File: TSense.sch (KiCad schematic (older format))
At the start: 52 parts, among them U10 LM393M, U11 LM393M, U2 LM393M, U3 LM393M, U4 LM393M, U5 LM393M, U6 LM393M, U7 LM393M, U8 LM393M, U9 LM393M

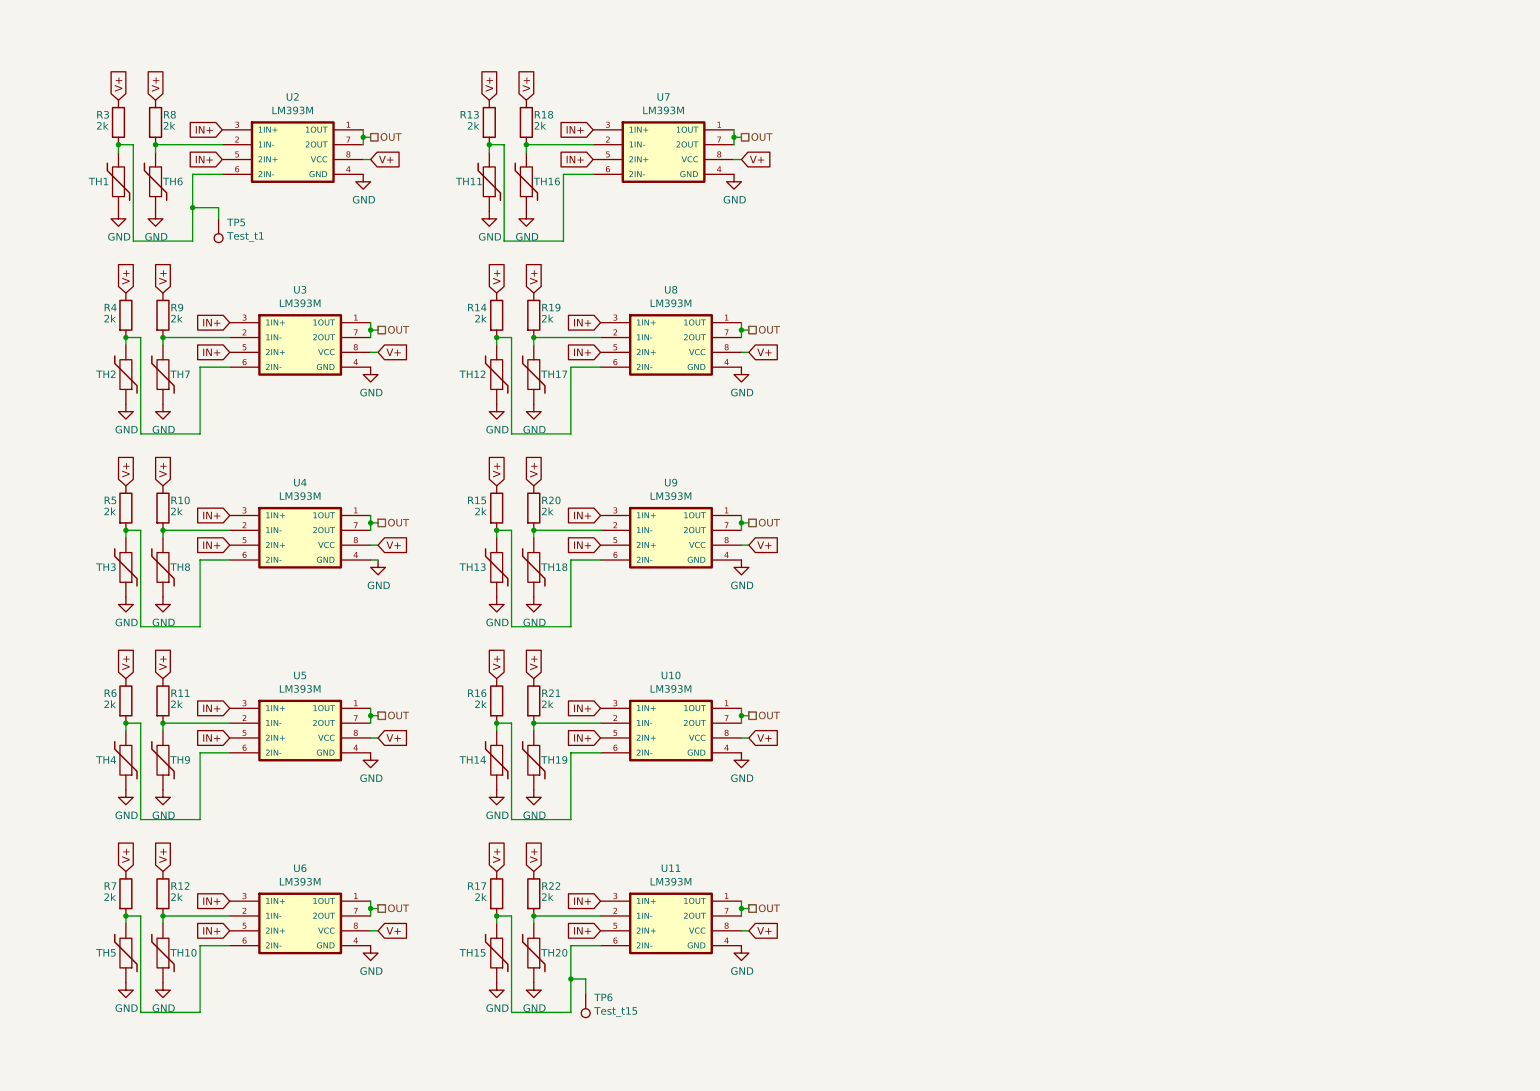
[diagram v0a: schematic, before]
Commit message: new
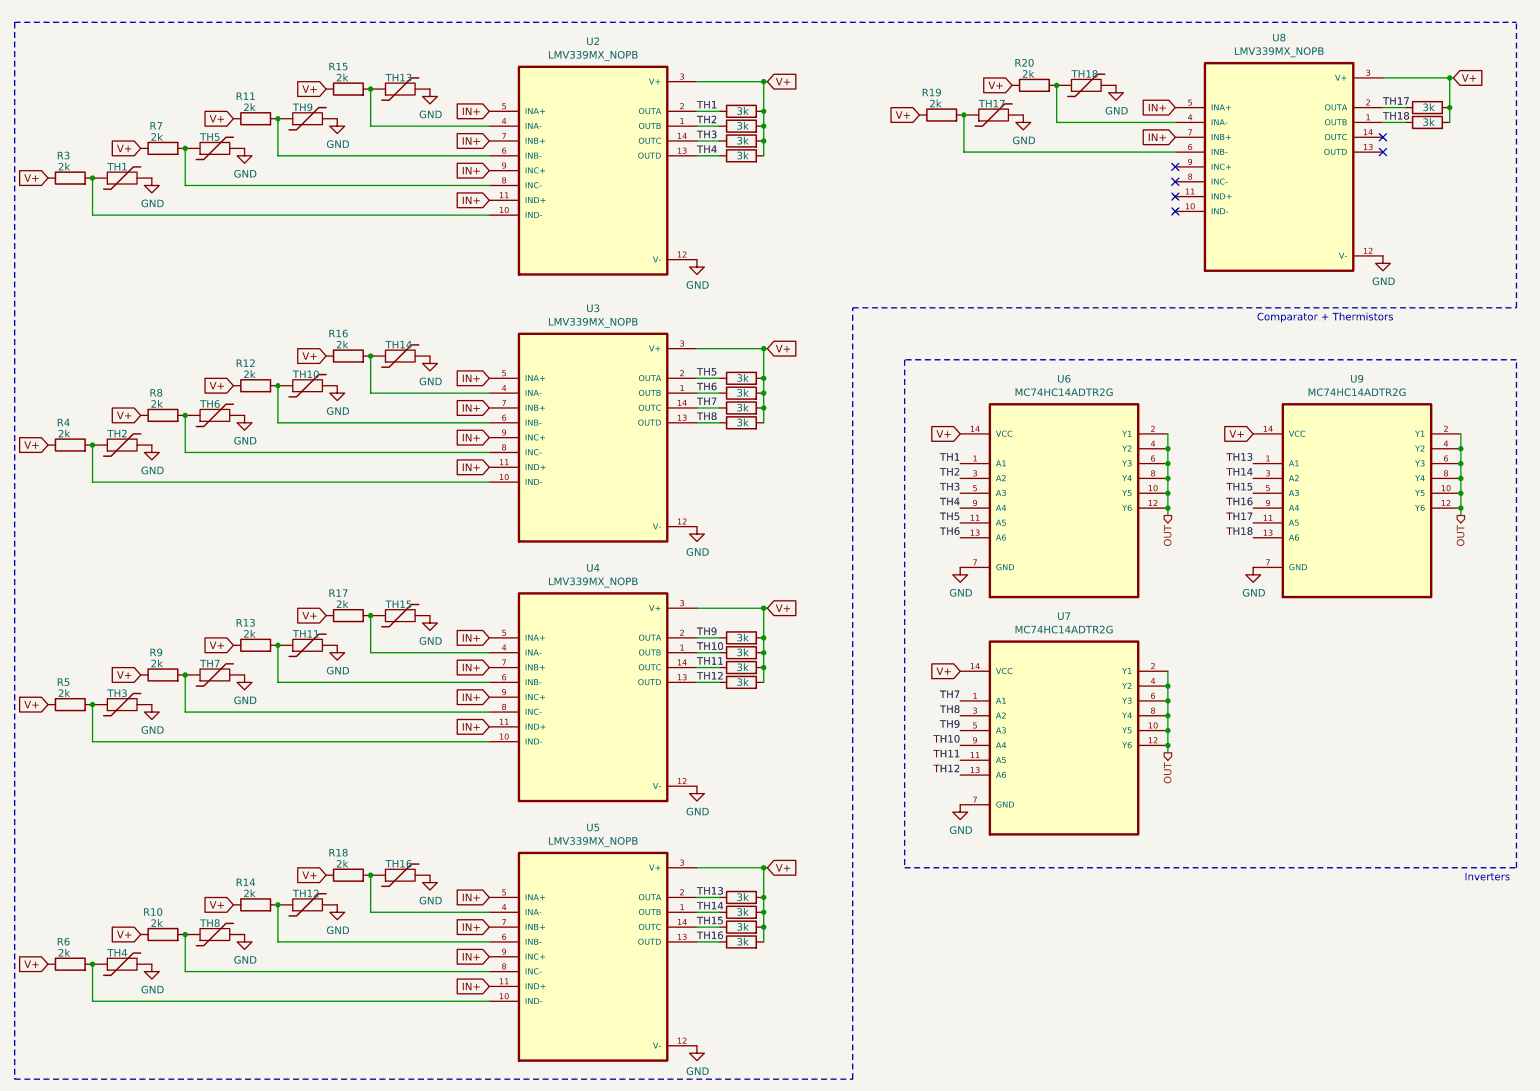
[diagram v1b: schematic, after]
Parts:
- removed R21, R22: 2k, Resistor_SMD:R_0805_2012Metric_Pad1.20x1.40mm_HandSolder, symbol Device:R
- removed TH19, TH20: 1k, Resistor_SMD:R_0603_1608Metric_Pad0.98x0.95mm_HandSolder, symbol Device:Thermistor
- removed TP5: Test_t1, LHRE Footprint Library:Test_Point_Tiny, symbol Connector:TestPoint
- removed TP6: Test_t15, LHRE Footprint Library:Test_Point_Tiny, symbol Connector:TestPoint
- removed U10, U11, U2, U3, U4, U5, U6, U7, U8, U9: LM393M, LHRE Footprint Library:SOIC127P599X175-8N, symbol Comparator:LM393DR
- added R? (x18): 3k, Resistor_SMD:R_0603_1608Metric_Pad0.98x0.95mm_HandSolder, symbol Device:R
- added U2, U3, U4, U5, U8: LMV339MX_NOPB, SOIC127P600X175-14N, symbol Comparator:LMV339MX_NOPB
- added U6, U7, U9: MC74HC14ADTR2G, LHRE Footprint Library:MC74HC14ADTR2G, symbol MC74HCT14ADG:MC74HC14ADTR2G
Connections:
- net GND: now also TH1.2, TH10.2, TH11.2, TH12.2, TH13.2, TH14.2, TH15.2, TH16.2, TH17.2, TH18.2, TH2.2, TH3.2, TH4.2, TH5.2, TH6.2, TH7.2, TH8.2, TH9.2, U2.12 (V-), U3.12 (V-), U4.12 (V-), U5.12 (V-), U6.7 (GND), U7.7 (GND), U8.12 (V-), U9.7 (GND); no longer TH1.1, TH10.1, TH11.1, TH12.1, TH13.1, TH14.1, TH15.1, TH16.1, TH17.1, TH18.1, TH2.1, TH3.1, TH4.1, TH5.1, TH6.1, TH7.1, TH8.1, TH9.1
- net IN+: now also U2.11 (IND+), U2.5 (INA+), U2.7 (INB+), U2.9 (INC+), U3.11 (IND+), U3.5 (INA+), U3.7 (INB+), U3.9 (INC+), U4.11 (IND+), U4.5 (INA+), U4.7 (INB+), U4.9 (INC+), U5.11 (IND+), U5.5 (INA+), U5.7 (INB+), U5.9 (INC+), U8.5 (INA+), U8.7 (INB+)
- net OUT: now also U6.10 (Y5), U6.12 (Y6), U6.2 (Y1), U6.4 (Y2), U6.6 (Y3), U6.8 (Y4), U7.10 (Y5), U7.12 (Y6), U7.2 (Y1), U7.4 (Y2), U7.6 (Y3), U7.8 (Y4), U9.10 (Y5), U9.12 (Y6), U9.2 (Y1), U9.4 (Y2), U9.6 (Y3), U9.8 (Y4)
- net V+: now also R?.2, R?.2, R?.2, R?.2, R?.2, R?.2, R?.2, R?.2, R?.2, R?.2, R?.2, R?.2, R?.2, R?.2, R?.2, R?.2, R?.2, R?.2, U2.3 (V+), U3.3 (V+), U4.3 (V+), U5.3 (V+), U6.14 (VCC), U7.14 (VCC), U8.3 (V+), U9.14 (VCC)
- net at R8.2: now also TH6.1, U3.8 (INC-); no longer TH6.2
- net at R3.2: now also TH1.1, U2.10 (IND-); no longer TH1.2
- net at R4.2: now also TH2.1, U3.10 (IND-); no longer TH2.2
- net at R9.2: now also TH7.1, U4.8 (INC-); no longer TH7.2
- net at R10.2: now also TH8.1, U5.8 (INC-); no longer TH8.2
- net at R5.2: now also TH3.1, U4.10 (IND-); no longer TH3.2
- net at R11.2: now also TH9.1, U2.6 (INB-); no longer TH9.2
- net at R6.2: now also TH4.1, U5.10 (IND-); no longer TH4.2
- net at R12.2: now also TH10.1, U3.6 (INB-); no longer TH10.2
- net at R7.2: now also TH5.1, U2.8 (INC-); no longer TH5.2
- net at R18.2: now also TH16.1, U5.4 (INA-); no longer TH16.2
- net at R13.2: now also TH11.1, U4.6 (INB-); no longer TH11.2
- net at R19.2: now also TH17.1, U8.6 (INB-); no longer TH17.2
- net at R14.2: now also TH12.1, U5.6 (INB-); no longer TH12.2
- net at R20.2: now also TH18.1, U8.4 (INA-); no longer TH18.2
- net at R15.2: now also TH13.1, U2.4 (INA-); no longer TH13.2
- net at R16.2: now also TH14.1, U3.4 (INA-); no longer TH14.2
- net at R17.2: now also TH15.1, U4.4 (INA-); no longer TH15.2
- new net TH1: R?.1, U2.2 (OUTA), U6.1 (A1)
- new net TH10: R?.1, U4.1 (OUTB), U7.9 (A4)
- new net TH11: R?.1, U4.14 (OUTC), U7.11 (A5)
- new net TH12: R?.1, U4.13 (OUTD), U7.13 (A6)
- new net TH13: R?.1, U5.2 (OUTA), U9.1 (A1)
- new net TH14: R?.1, U5.1 (OUTB), U9.3 (A2)
- new net TH15: R?.1, U5.14 (OUTC), U9.5 (A3)
- new net TH16: R?.1, U5.13 (OUTD), U9.9 (A4)
- new net TH17: R?.1, U8.2 (OUTA), U9.11 (A5)
- new net TH18: R?.1, U8.1 (OUTB), U9.13 (A6)
- new net TH2: R?.1, U2.1 (OUTB), U6.3 (A2)
- new net TH3: R?.1, U2.14 (OUTC), U6.5 (A3)
- new net TH4: R?.1, U2.13 (OUTD), U6.9 (A4)
- new net TH5: R?.1, U3.2 (OUTA), U6.11 (A5)
- new net TH6: R?.1, U3.1 (OUTB), U6.13 (A6)
- new net TH7: R?.1, U3.14 (OUTC), U7.1 (A1)
- new net TH8: R?.1, U3.13 (OUTD), U7.3 (A2)
- new net TH9: R?.1, U4.2 (OUTA), U7.5 (A3)
- no-connect marks 0 -> 6
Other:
- note added: "Comparator + Thermistors\n"
- note added: "Inverters\n"

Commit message: Add files via upload
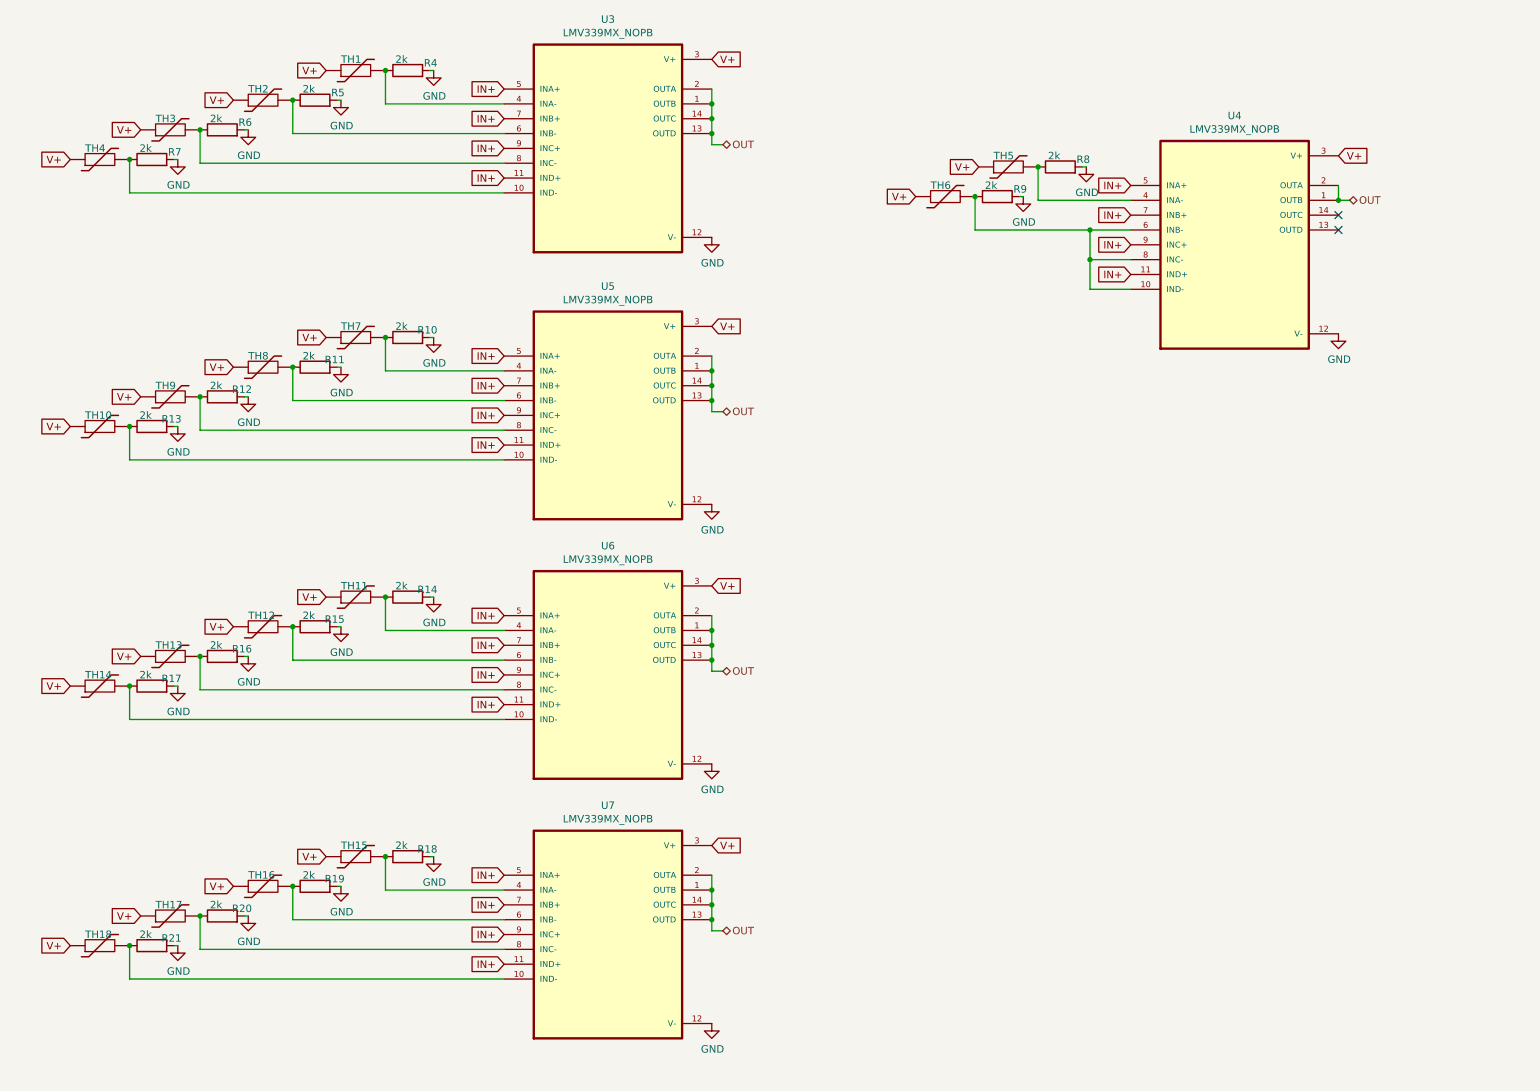
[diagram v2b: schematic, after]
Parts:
- removed R7: 2k, Resistor_SMD:R_0805_2012Metric_Pad1.20x1.40mm_HandSolder, symbol Device:R
- removed R? (x18): 3k, Resistor_SMD:R_0603_1608Metric_Pad0.98x0.95mm_HandSolder, symbol Device:R
- removed TH4: 1k, Resistor_SMD:R_0603_1608Metric_Pad0.98x0.95mm_HandSolder, symbol Device:Thermistor
- removed U6, U7, U9: MC74HC14ADTR2G, LHRE Footprint Library:MC74HC14ADTR2G, symbol MC74HCT14ADG:MC74HC14ADTR2G
- added R21: 2k, Resistor_SMD:R_0805_2012Metric_Pad1.20x1.40mm_HandSolder, symbol Device:R
- added TH1: 1k, Resistor_SMD:R_1206_3216Metric_Pad1.30x1.75mm_HandSolder, symbol Device:Thermistor
- TH10, TH11, TH12, TH13, TH14, TH15, TH16, TH17, TH18, TH2, TH3, TH5, TH6, TH7, TH8, TH9: footprint Resistor_SMD:R_0603_1608Metric_Pad0.98x0.95mm_HandSolder -> Resistor_SMD:R_1206_3216Metric_Pad1.30x1.75mm_HandSolder
- TH4: renamed from TH1; footprint Resistor_SMD:R_0603_1608Metric_Pad0.98x0.95mm_HandSolder -> Resistor_SMD:R_1206_3216Metric_Pad1.30x1.75mm_HandSolder
- renumbered R3 to R7, U2 to U3, U8 to U4, U3 to U5, U4 to U6, U5 to U7
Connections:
- net TH1 is gone; now on net OUT: U3.2 (OUTA)
- net TH10 is gone; now on net OUT: U6.1 (OUTB)
- net TH11 is gone; now on net OUT: U6.14 (OUTC)
- net TH12 is gone; now on net OUT: U6.13 (OUTD)
- net TH13 is gone; now on net OUT: U7.2 (OUTA)
- net TH14 is gone; now on net OUT: U7.1 (OUTB)
- net TH15 is gone; now on net OUT: U7.14 (OUTC)
- net TH16 is gone; now on net OUT: U7.13 (OUTD)
- net TH17 is gone; now on net OUT: U4.2 (OUTA)
- net TH18 is gone; now on net OUT: U4.1 (OUTB)
- net TH2 is gone; now on net OUT: U3.1 (OUTB)
- net TH3 is gone; now on net OUT: U3.14 (OUTC)
- net TH4 is gone; now on net OUT: U3.13 (OUTD)
- net TH5 is gone; now on net OUT: U5.2 (OUTA)
- net TH6 is gone; now on net OUT: U5.1 (OUTB)
- net TH7 is gone; now on net OUT: U5.14 (OUTC)
- net TH8 is gone; now on net OUT: U5.13 (OUTD)
- net TH9 is gone; now on net OUT: U6.2 (OUTA)
- net GND: now also R10.2, R11.2, R12.2, R13.2, R14.2, R15.2, R16.2, R17.2, R18.2, R19.2, R20.2, R4.2, R5.2, R6.2, R7.2, R8.2, R9.2, R21.2; no longer TH10.2, TH11.2, TH12.2, TH13.2, TH14.2, TH15.2, TH16.2, TH17.2, TH18.2, TH2.2, TH3.2, TH4.2, TH5.2, TH6.2, TH7.2, TH8.2, TH9.2
- net IN+: now also U4.11 (IND+), U4.9 (INC+)
- net V+: now also TH10.1, TH11.1, TH12.1, TH13.1, TH14.1, TH15.1, TH16.1, TH17.1, TH18.1, TH2.1, TH3.1, TH4.1, TH5.1, TH6.1, TH7.1, TH8.1, TH9.1, TH1.1; no longer R10.1, R11.1, R12.1, R13.1, R14.1, R15.1, R16.1, R17.1, R18.1, R19.1, R20.1, R4.1, R5.1, R6.1, R7.1, R8.1, R9.1
- net at U3.8 (INC-): now also R6.1, TH3.2; no longer TH5.1
- net at U7.10 (IND-): now also TH18.2, R21.1; no longer R6.2
- net at U4.10 (IND-): now also R9.1, TH6.2, U4.6 (INB-), U4.8 (INC-)
- new net: R7.1, TH4.2, U3.10 (IND-)
- new net: R4.1, TH1.2, U3.4 (INA-)
- new net: R5.1, TH2.2, U3.6 (INB-)
- new net: R13.1, TH10.2, U5.10 (IND-)
- new net: R10.1, TH7.2, U5.4 (INA-)
- new net: R11.1, TH8.2, U5.6 (INB-)
- new net: R12.1, TH9.2, U5.8 (INC-)
- new net: R17.1, TH14.2, U6.10 (IND-)
- new net: R14.1, TH11.2, U6.4 (INA-)
- new net: R15.1, TH12.2, U6.6 (INB-)
- new net: R16.1, TH13.2, U6.8 (INC-)
- new net: R18.1, TH15.2, U7.4 (INA-)
- new net: R19.1, TH16.2, U7.6 (INB-)
- new net: R20.1, TH17.2, U7.8 (INC-)
- new net: R8.1, TH5.2, U4.4 (INA-)
- no-connect marks 6 -> 2
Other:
- note removed: "Comparator + Thermistors\n"
- note removed: "Inverters\n"
- moved on the sheet: R7, TH4, U3, U4, U5, U6, U7
